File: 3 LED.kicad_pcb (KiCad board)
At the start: 2 copper layers, 24 x 48.8 mm, 22 parts, among them J1 Conn_01x04_Socket, Q1 NPN, Q2 NPN, Q3 NPN, U1 74HC238D

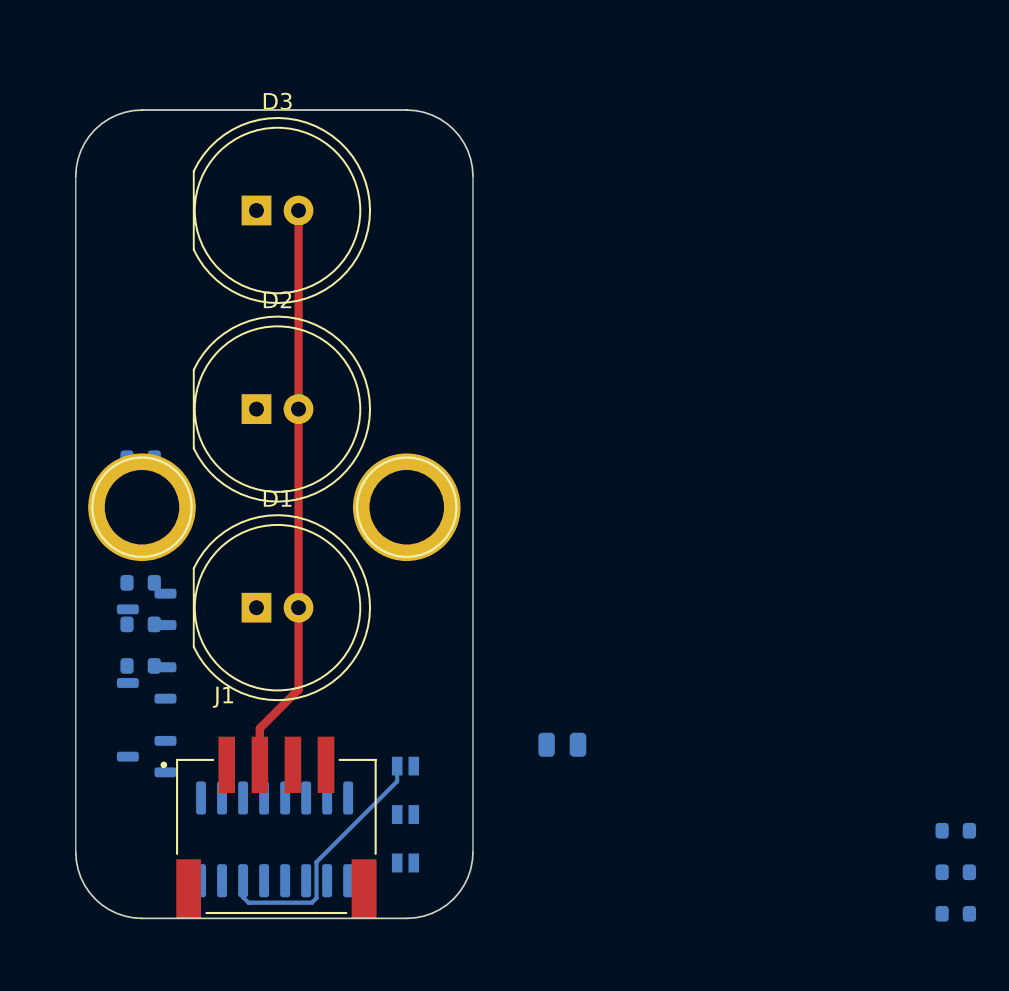
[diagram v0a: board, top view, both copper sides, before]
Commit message: Production V2
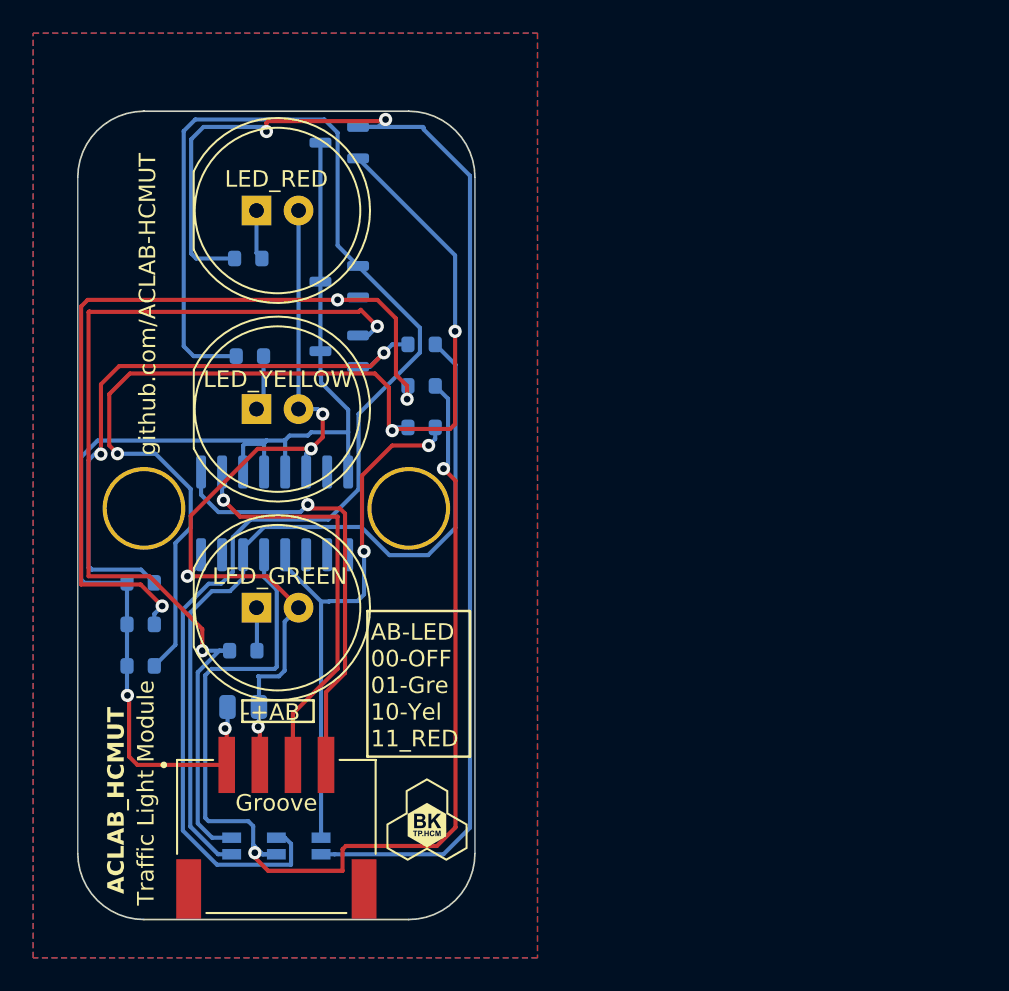
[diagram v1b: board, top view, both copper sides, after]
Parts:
- removed the REF** at (142.5, 116.0)
- added G***: LOGO, DeltaKiteEngineering:BKU_Medium, F.Cu at (150.8, 128.8)
- added REF**: Ohstem_Base, ACLAB:Ohstem_Base_V2, F.Cu at (142.6, 116.1)
- moved R5 43.7 mm to (150.5, 102.6)
- moved R6 43.7 mm to (150.5, 105.1)
- moved R4 43.7 mm to (150.5, 100.1)
- moved Q3 38.9 mm to (145.5, 87.9)
- moved Q2 26.9 mm to (145.5, 96.3)
- moved U1 19.7 mm to (141.6, 110.3)
- moved Q1 19.5 mm to (145.5, 100.5)
- moved C1 19.4 mm to (139.7, 122.0)
- moved R3 18.3 mm to (140.0, 94.9)
- moved R1 13.2 mm to (139.7, 118.6)
- moved JP1 11.6 mm to (139.0, 130.4), turned to -90 degrees
- moved R2 10.9 mm to (140.1, 100.8)
- moved JP2 8.03 mm to (141.7, 130.4), turned to -90 degrees
- moved JP3 5.20 mm to (144.4, 130.4), turned to -90 degrees
- renumbered J1 to Groove, D1 to LED_GREEN, D3 to LED_RED, D2 to LED_YELLOW
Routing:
- net Net-(JP2-A): track 0.00 -> 89.4 mm
- net Net-(JP3-B): track 0.00 -> 81.5 mm, vias 0 -> 2
- net GND: track 0.00 -> 74.9 mm, vias 0 -> 2
- net /L2: track 0.00 -> 70.0 mm, vias 0 -> 2
- net Net-(Q3-B): track 0.00 -> 64.7 mm, vias 0 -> 3
- net Net-(JP1-A): track 0.00 -> 60.4 mm, vias 0 -> 2
- net Net-(Q2-B): track 0.00 -> 50.5 mm, vias 0 -> 3
- net Net-(Q1-B): track 0.00 -> 37.8 mm, vias 0 -> 2
- net /L3: track 0.00 -> 34.0 mm, vias 0 -> 2
- net /L1: track 15.7 -> 48.3 mm
- net /S0: track 0.00 -> 26.7 mm, vias 0 -> 1
- net /S1: track 0.00 -> 25.2 mm, vias 0 -> 1
- net +5V: track 34.5 -> 50.7 mm, vias 0 -> 4
- net Net-(D2-K): track 0.00 -> 3.38 mm
- net Net-(D3-K): track 0.00 -> 3.03 mm
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- added copper zone on B.Cu, net GND
- added copper zone on F.Cu, net GND
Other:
- board text added: "-+AB"
- board text added: "AB-LED 00-OFF 01-Gre 10-Yel 11_RED"
- board text added: "ACLAB_HCMUT"
- board text added: "Traffic Light Module"
- board text added: "github.com/ACLAB-HCMUT"
